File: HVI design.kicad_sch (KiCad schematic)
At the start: 24 parts, among them Q1 TK3P80E, U1 LT8316EFE, U2 TLV1702

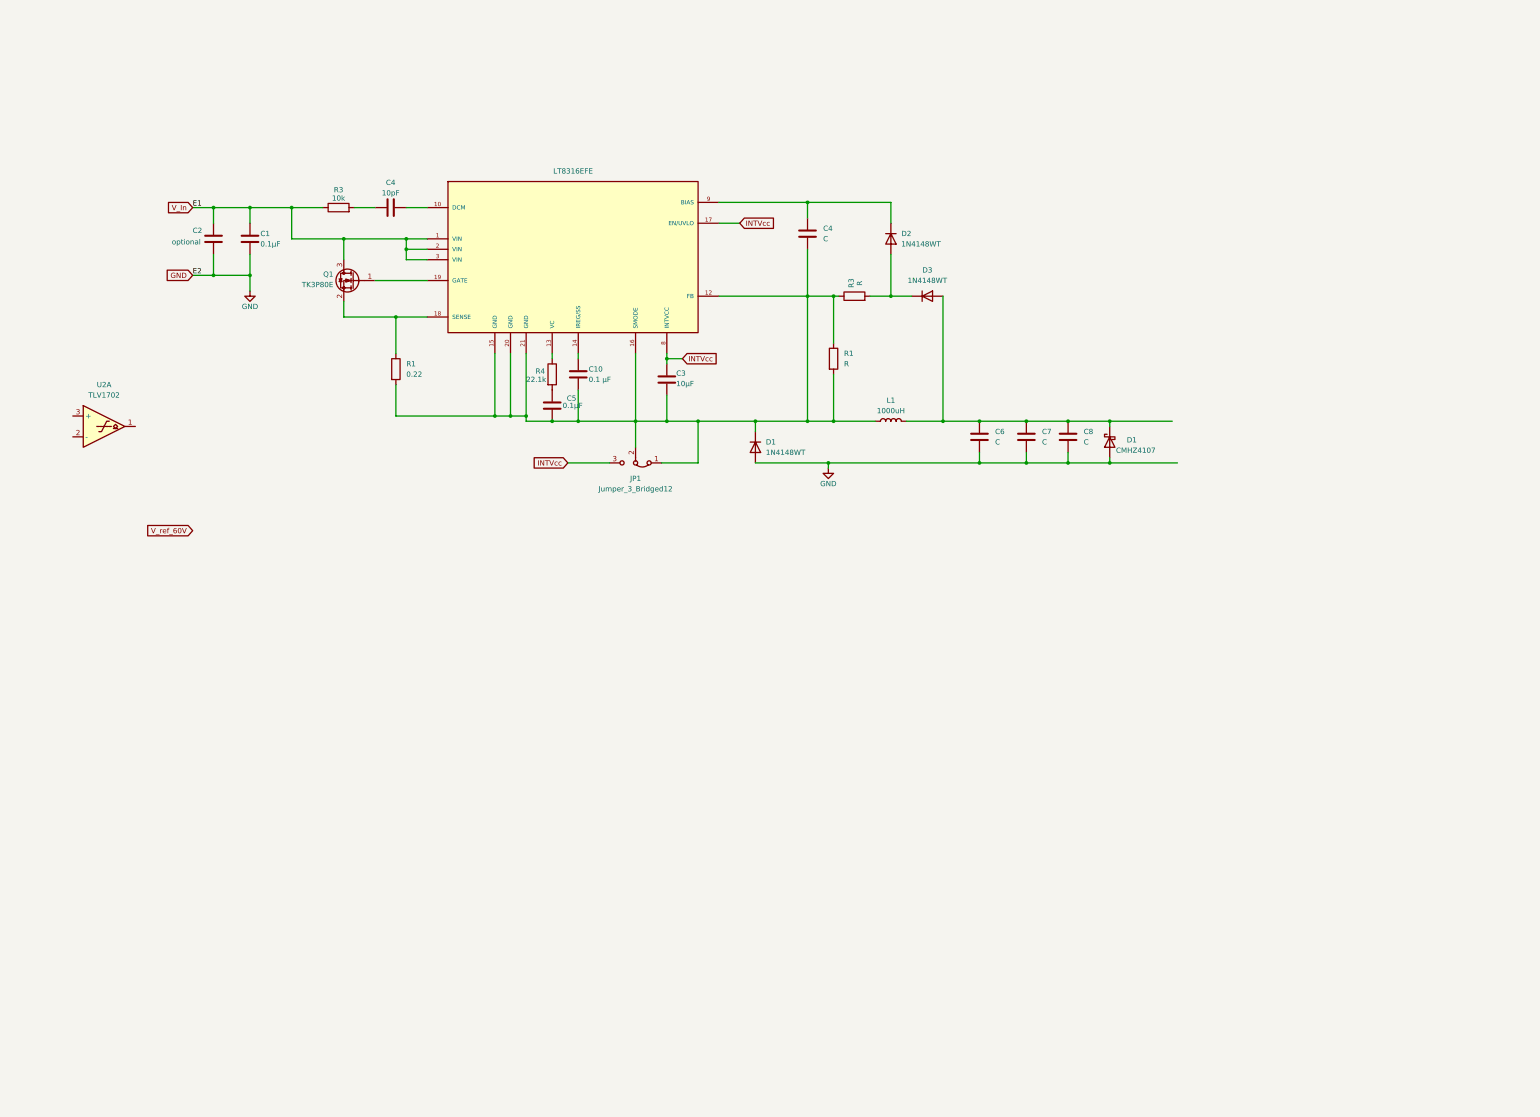
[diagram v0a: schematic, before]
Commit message: Add files via upload
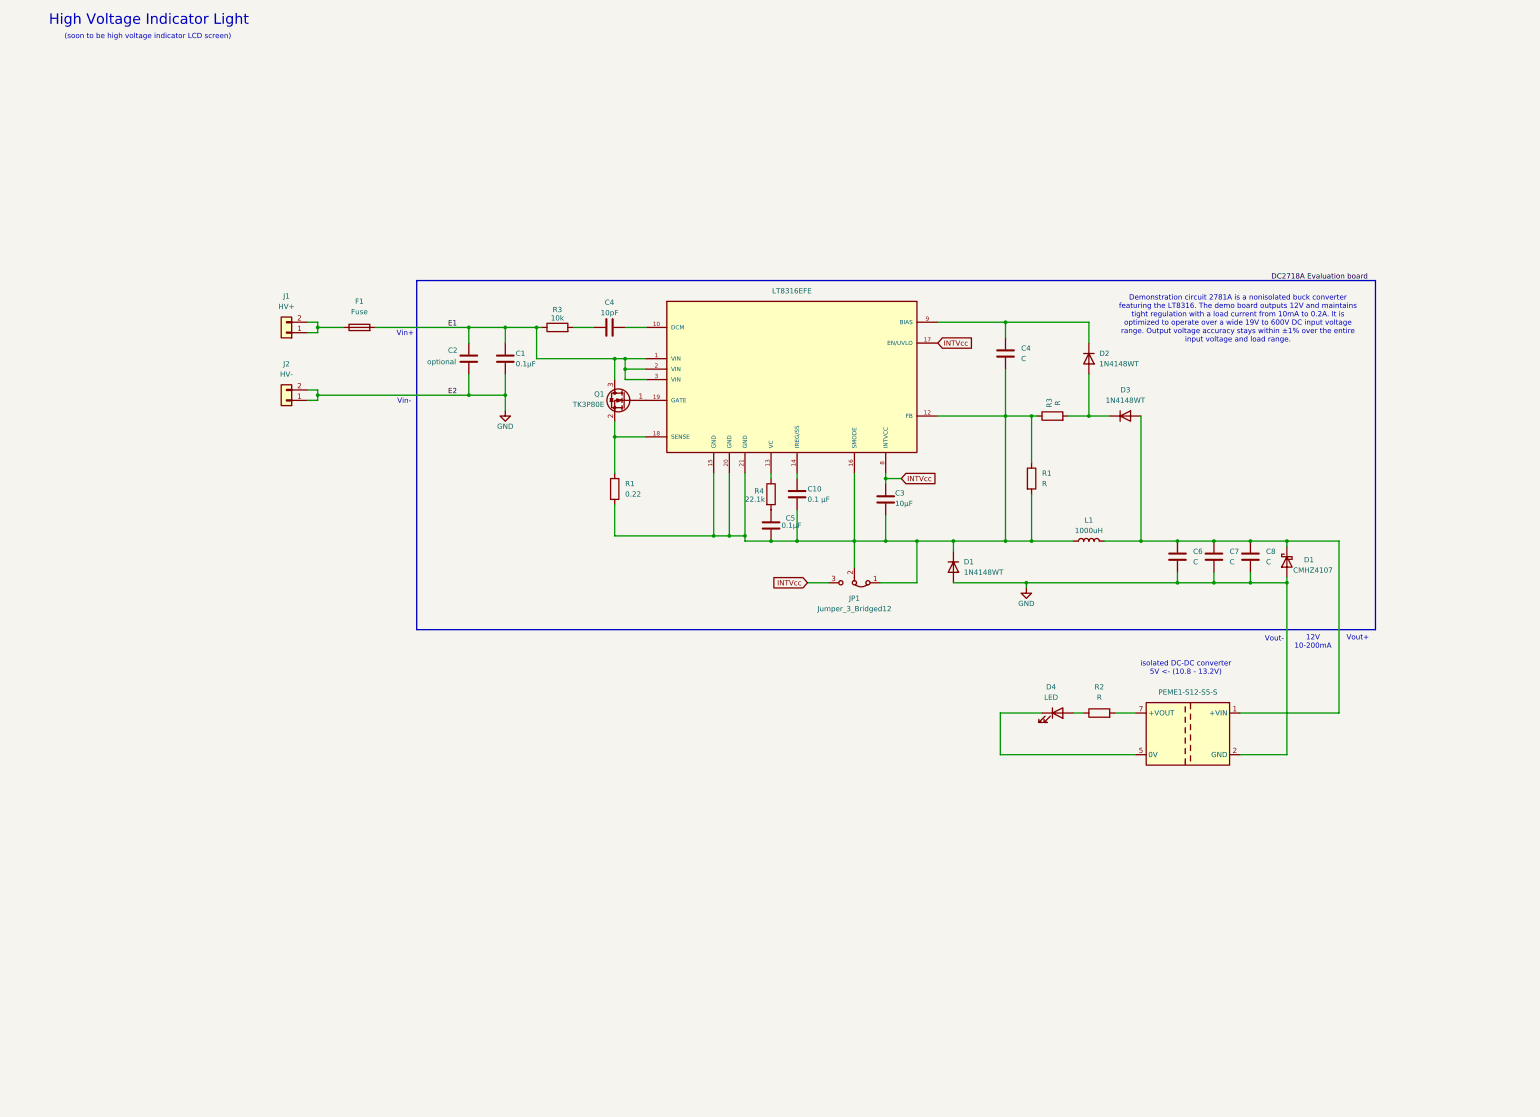
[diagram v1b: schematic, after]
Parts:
- removed U2: TLV1702, Custom_MSM:Comparator_Dual_VSSOP-8, symbol Custom_MSM:Comparator_Dual_Open-Coll
- added D4: LED, symbol Device:LED
- added F1: Fuse, symbol Device:Fuse
- added J1: HV+, Custom_MSM:Connector_PP15, symbol Custom_MSM:Connector_PP15
- added J2: HV-, Custom_MSM:Connector_PP15, symbol Custom_MSM:Connector_PP15
- added R2: R, symbol Device:R
- added U3: PEME1-S12-S5-S, Converter_DCDC:Converter_DCDC_Murata_CRE1xxxxxxSC_THT, symbol Regulator_Switching:CRE1S1205SC
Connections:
- net GND: now also J2.1 (Pin_1), J2.2 (Pin_2), U3.2 (GND)
- net at C6.1, C7.1, C8.1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: now also U3.1 (+VIN)
- net V_In renamed E1
- net E1: now also F1.2
- new net: F1.1, J1.1 (Pin_1), J1.2 (Pin_2)
- new net: D4.2 (A), R2.1
- new net: R2.2, U3.7 (+VOUT)
- new net: D4.1 (K), U3.5 (0V)
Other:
- note added: "(soon to be high voltage indicator LCD screen)"
- note added: "12V 10-200mA"
- note added: "Demonstration circuit 2781A is a nonisolated buck converter featuring the LT8316. The demo board outputs 12V and maintains tight regulation with a load current from 10mA to 0.2A. It is optimized to operate over a wide 19V to 600V DC input voltage range. Output voltage accuracy stays within ±1% over the entire input voltage and load range."
- note added: "High Voltage Indicator Light"
- note added: "Vin+"
- note added: "Vin-"
- note added: "Vout+"
- note added: "Vout-"
- note added: "isolated DC-DC converter 5V <- (10.8 - 13.2V)"
- title: (none) -> High Voltage Indicator Light FS2026 EV
- moved on the sheet: C1, C10, C2, C3, C4, C5, C6, C7, C8, D1, D2, D3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

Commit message: Add files via upload
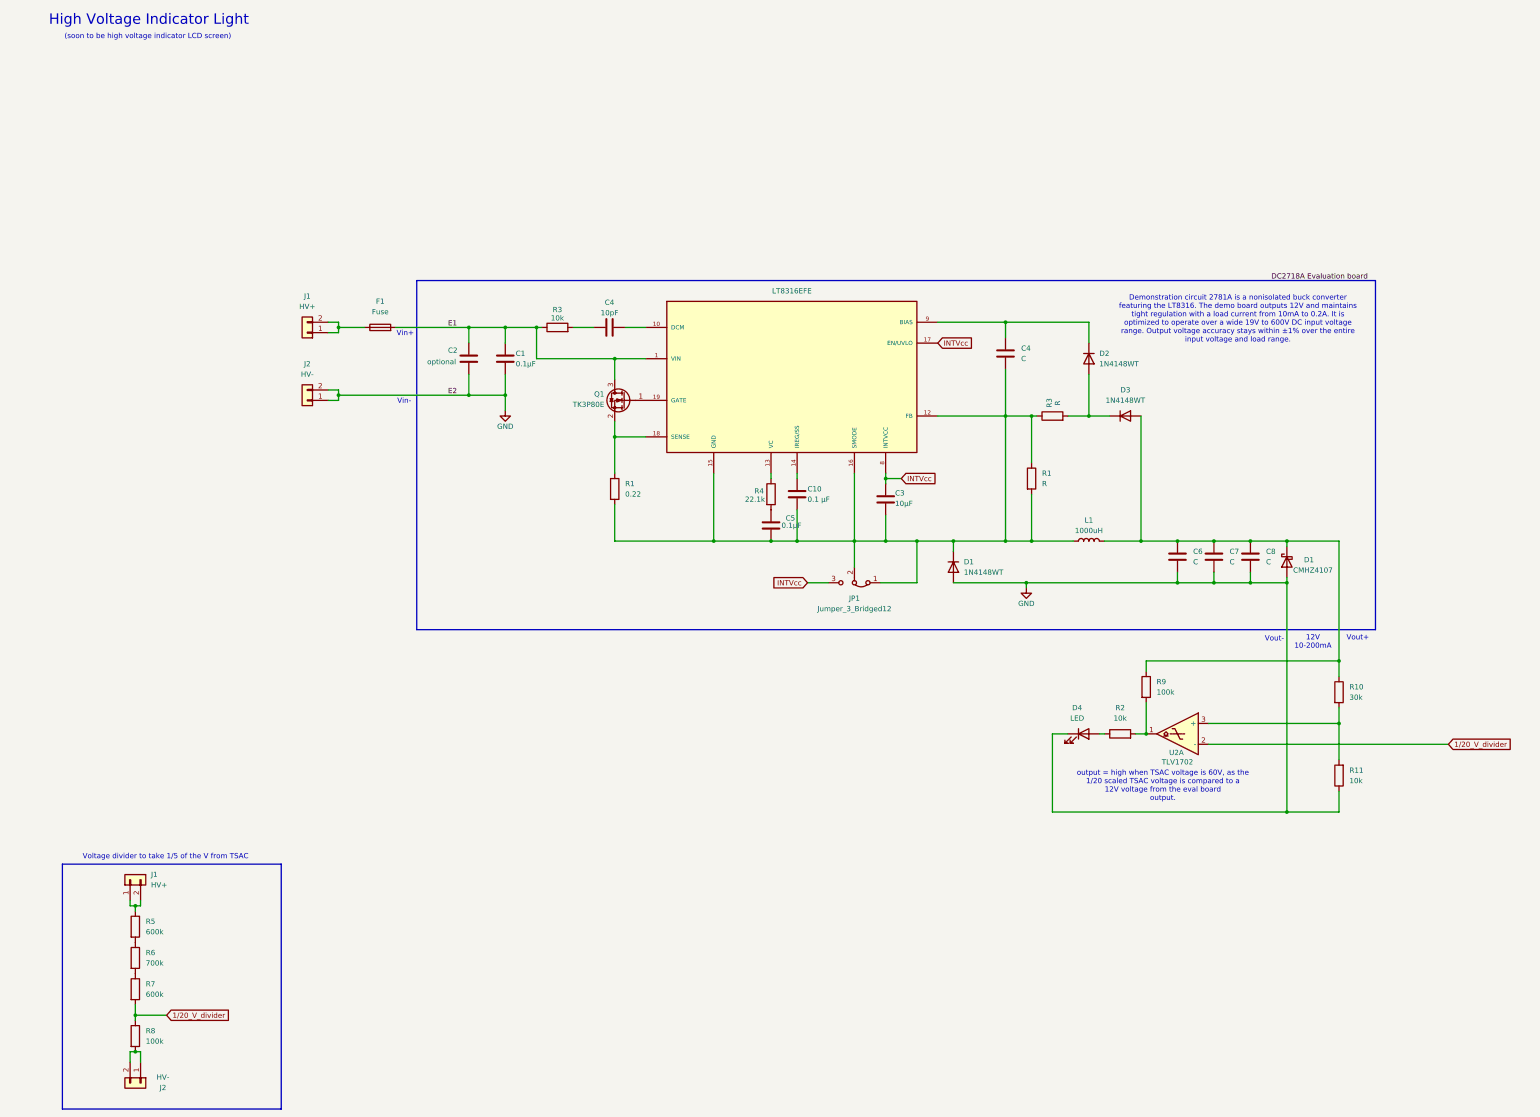
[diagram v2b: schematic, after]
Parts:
- removed U3: PEME1-S12-S5-S, Converter_DCDC:Converter_DCDC_Murata_CRE1xxxxxxSC_THT, symbol Regulator_Switching:CRE1S1205SC
- added J1: HV+, Custom_MSM:Connector_PP15, symbol Custom_MSM:Connector_PP15
- added J2: HV-, Custom_MSM:Connector_PP15, symbol Custom_MSM:Connector_PP15
- added R10: 30k, symbol Device:R
- added R11: 10k, symbol Device:R
- added R5, R7: 600k, symbol Device:R
- added R6: 700k, symbol Device:R
- added R8, R9: 100k, symbol Device:R
- added U2: TLV1702, Custom_MSM:Comparator_Dual_VSSOP-8, symbol Custom_MSM:Comparator_Dual_Open-Coll
- R2: value R -> 10k
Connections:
- net GND: now also D4.1 (K), R11.1
- net at C6.1, C7.1, C8.1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: now also R10.1, R9.1
- net at R2.2: now also R9.2, U2.1
- new net: R6.2, R7.1
- new net: R10.2, R11.2, U2.3 (+)
- new net: J2.1 (Pin_1), J2.2 (Pin_2), R8.2
- new net: R5.2, R6.1
- new net: U1.2 (VIN), U1.3 (VIN) (x2)
- new net: J1.1 (Pin_1), J1.2 (Pin_2), R5.1
- new net 1/20_V_divider: R7.2, R8.1, U2.2 (-)
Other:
- note added: "Voltage divider to take 1/5 of the V from TSAC"
- note added: "output = high when TSAC voltage is 60V, as the 1/20 scaled TSAC voltage is compared to a 12V voltage from the eval board output."
- note removed: "isolated DC-DC converter 5V <- (10.8 - 13.2V)"
- moved on the sheet: F1, J1, J2
